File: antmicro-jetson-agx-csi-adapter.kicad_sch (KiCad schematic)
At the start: 0 parts

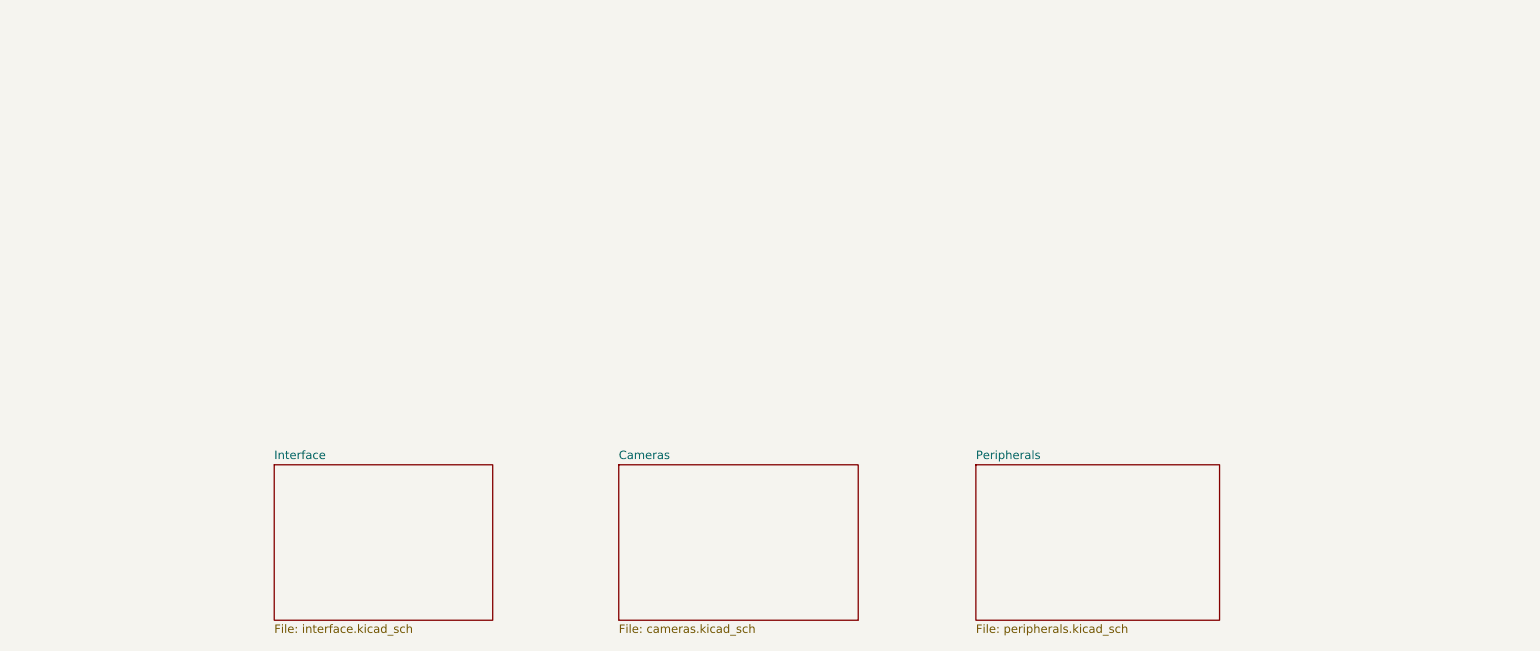
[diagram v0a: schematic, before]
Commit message: More changes from review
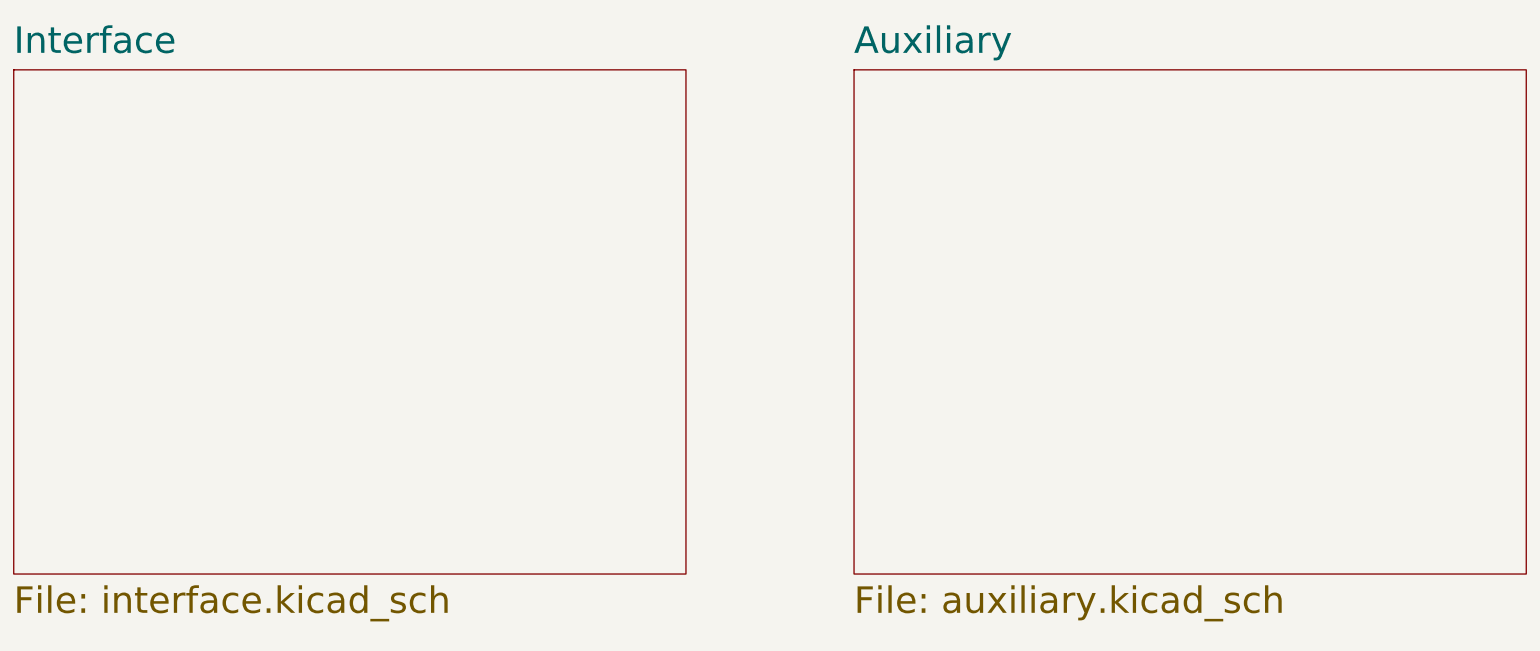
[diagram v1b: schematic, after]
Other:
- sheet Cameras renamed Auxiliary
- removed sheet Peripherals
- sheet Auxiliary: file cameras.kicad_sch -> auxiliary.kicad_sch

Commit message: Add TVS to wire connectors
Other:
- title: (none) -> Antmicro Jetson AGX CSI Adapter
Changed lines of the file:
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@@
   (paper "A3")
   (title_block
+    (title "Antmicro Jetson AGX CSI Adapter")
     (date "2022-07-20")
     (rev "1.0.0")
@@
       (reference "#PWR?") (unit 1) (value "GND") (footprint "")
     )
+    (path "/979ab030-ea70-442d-80da-03811f49b178/11863630-b44b-4338-9bc6-aa72492c71bb"
+      (reference "#PWR?") (unit 1) (value "GND") (footprint "")
+    )
     (path "/979ab030-ea70-442d-80da-03811f49b178/1867d3f7-d6b3-49ee-9356-dde2de938418"
+      (reference "#PWR?") (unit 1) (value "GND") (footprint "")
+    )
+    (path "/979ab030-ea70-442d-80da-03811f49b178/1d232c02-d38c-4627-a499-27091666a11e"
       (reference "#PWR?") (unit 1) (value "GND") (footprint "")
     )
@@
       (reference "#PWR?") (unit 1) (value "GND") (footprint "")
     )
+    (path "/979ab030-ea70-442d-80da-03811f49b178/9305c781-5e20-439a-9f8f-c0f1fad558b1"
+      (reference "#PWR?") (unit 1) (value "GND") (footprint "")
+    )
     (path "/979ab030-ea70-442d-80da-03811f49b178/957db8d9-d72f-41ab-9014-0289cdf92576"
       (reference "#PWR?") (unit 1) (value "+3V3") (footprint "")
@@
       (reference "D?") (unit 1) (value "LTST-C190GKT") (footprint "antmicro-footprints:LED_0603")
     )
+    (path "/979ab030-ea70-442d-80da-03811f49b178/611f77ae-ee8c-40d5-8ef0-80ff1e328d46"
+      (reference "D?") (unit 1) (value "PUSB3F96X_PASS") (footprint "antmicro-footprints:PUSB3F96X")
+    )
+    (path "/979ab030-ea70-442d-80da-03811f49b178/77638668-2257-4b6d-838d-16e976f4f331"
+      (reference "D?") (unit 1) (value "PUSB3F96X_PASS") (footprint "antmicro-footprints:PUSB3F96X")
+    )
     (path "/62c966ae-f4cc-414f-ab0e-87e058efb422/77eed193-2eb1-4f15-956a-ee4c267cb676"
       (reference "D?") (unit 1) (value "LTST-C190GKT") (footprint "antmicro-footprints:LED_0603")
@@
       (reference "D?") (unit 1) (value "LTST-C190GKT") (footprint "antmicro-footprints:LED_0603")
     )
+    (path "/979ab030-ea70-442d-80da-03811f49b178/dd8bfae5-2d6b-499c-9e30-5b97e97a485e"
+      (reference "D?") (unit 1) (value "PUSB3F96X_PASS") (footprint "antmicro-footprints:PUSB3F96X")
+    )
     (path "/62c966ae-f4cc-414f-ab0e-87e058efb422/f3b063d9-d372-4ff8-b46c-39fa68ea5928"
